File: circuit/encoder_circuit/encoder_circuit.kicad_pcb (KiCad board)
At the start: 2 copper layers, 2.5 x 2.6 mm, 6 parts, among them J1 Conn_01x04

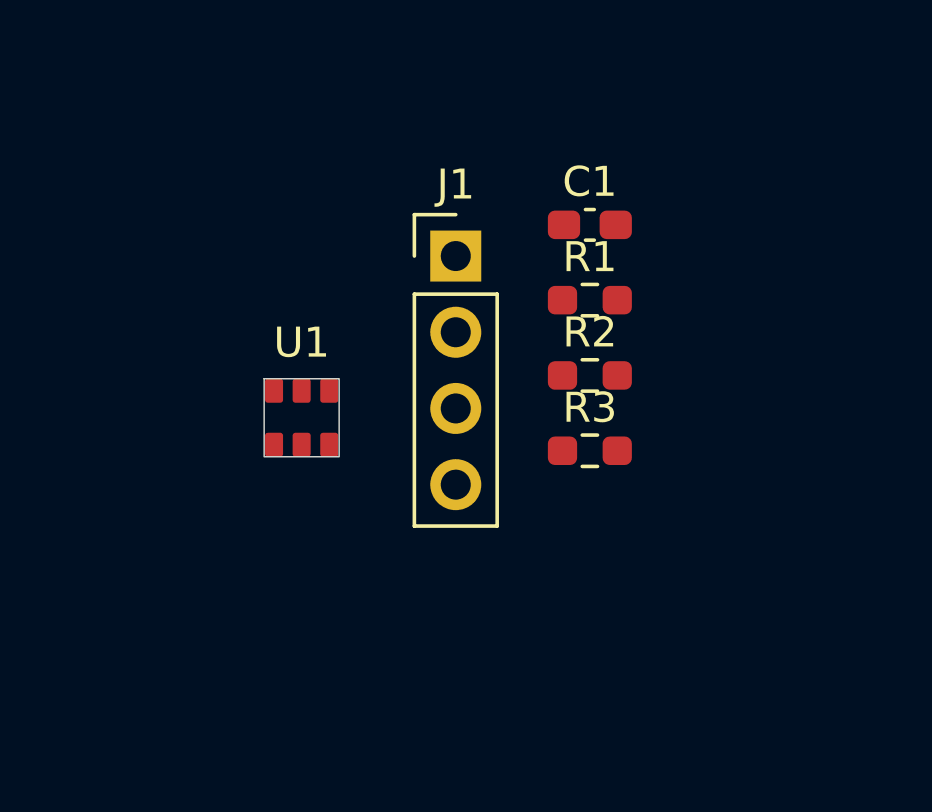
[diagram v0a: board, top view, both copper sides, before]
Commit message: step
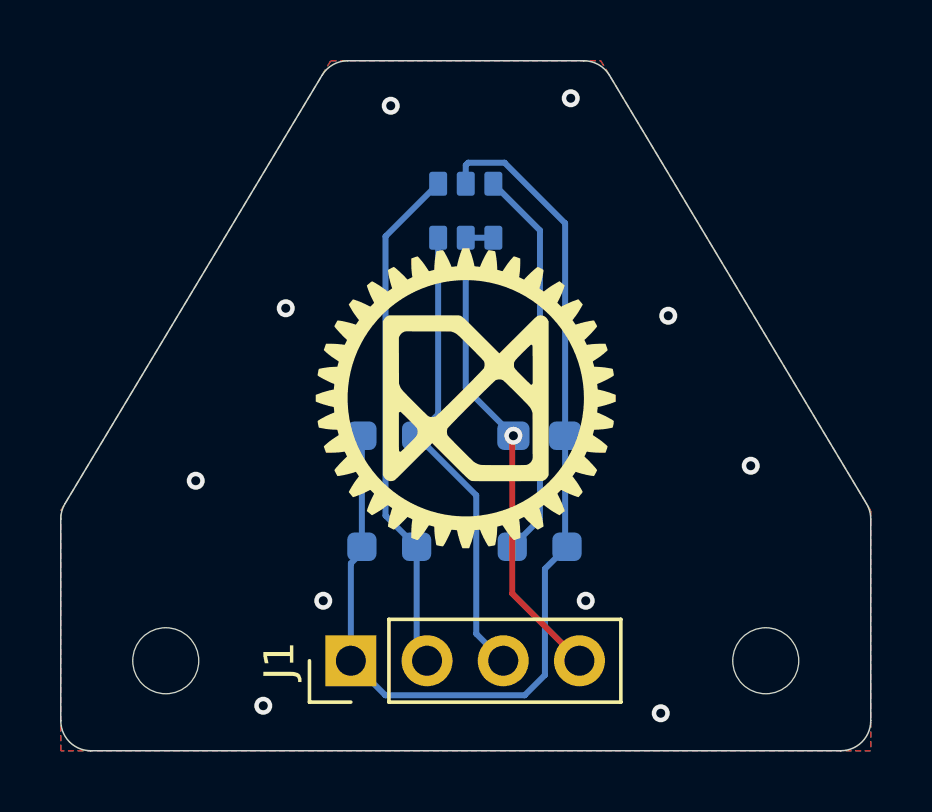
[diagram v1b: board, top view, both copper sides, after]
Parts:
- added G***: LOGO, Symbol:sh_10mm, F.Cu at (141.8, 92.2)
- added REF**: MountingHole_2.2mm_M2, MountingHole:MountingHole_2.2mm_M2, F.Cu at (131.8, 101.0)
- added REF**: MountingHole_2.2mm_M2, MountingHole:MountingHole_2.2mm_M2, F.Cu at (151.8, 101.0)
- C1, R1, R2, R3, U1: moved to B.Cu
- moved J1 13.9 mm to (137.9, 101.0), turned to 90 degrees
- moved U1 8.81 mm to (141.8, 86.0), turned to 180 degrees
- moved R2 8.79 mm to (139.2, 97.2)
- moved R1 8.39 mm to (144.2, 97.2), turned to 180 degrees
- moved C1 7.23 mm to (144.2, 93.5), turned to 180 degrees
- moved R3 6.71 mm to (139.2, 93.5)
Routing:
- net +3.3V: track 0.00 -> 35.1 mm
- net Net-(J1-Pin_2): track 0.00 -> 17.2 mm
- net GND: track 0.00 -> 16.6 mm, vias 0 -> 11
- net Net-(J1-Pin_3): track 0.00 -> 15.6 mm
- net Net-(U1-Anode): track 0.00 -> 13.1 mm
- added copper zone on B.Cu, net GND
- added copper zone on F.Cu, net GND
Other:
- board size 2.5 x 2.6 mm -> 27 x 23 mm
